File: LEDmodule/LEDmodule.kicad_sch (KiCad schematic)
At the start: 2 parts

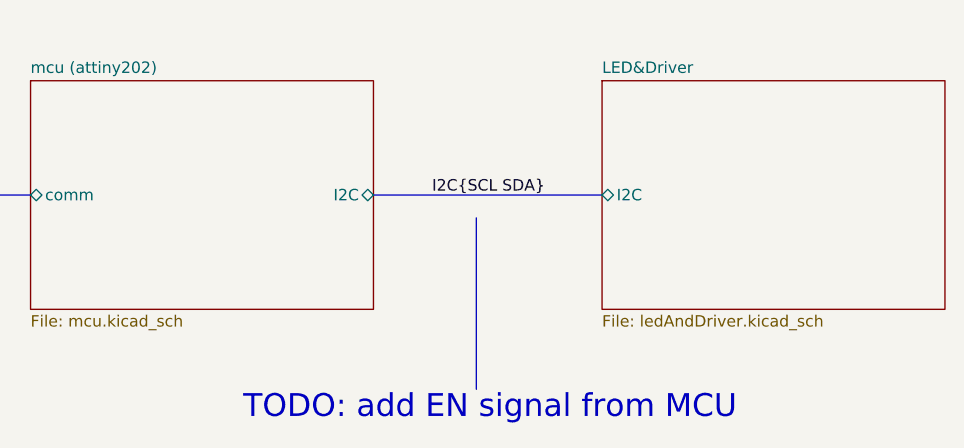
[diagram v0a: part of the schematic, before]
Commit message: Finalize Led&Driver
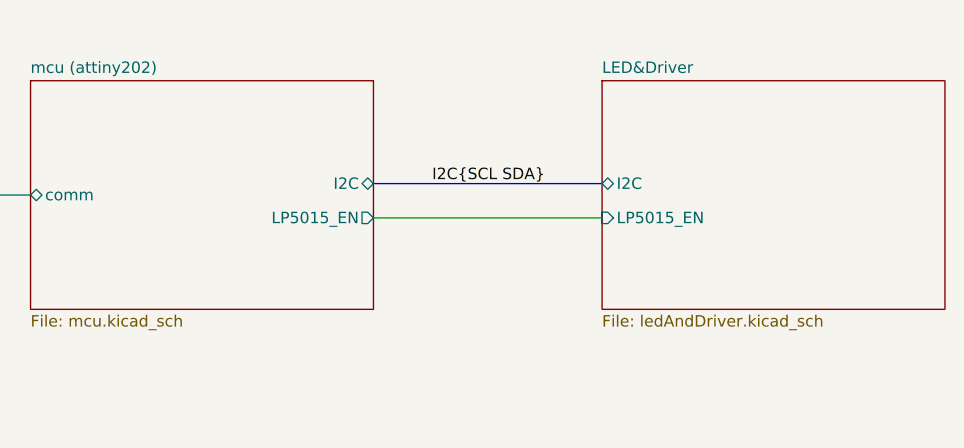
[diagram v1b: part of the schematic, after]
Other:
- sheet LED&Driver ports: added LP5015_EN; removed none
- sheet mcu (attiny202) ports: added LP5015_EN; removed none
- note removed: "TODO: add EN signal from MCU"
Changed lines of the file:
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@@
 		(comment 1 "${Designed By}")
-	)
-	(text "TODO: add EN signal from MCU"
-		(exclude_from_sim no)
-		(at 228.854 150.622 0)
-		(effects
-			(font
-				(size 2.54 2.54)
-				(color 255 0 0 1)
-			)
-		)
 	)
 	(junction
@@
 	(bus
 		(pts
-			(xy 215.9 127) (xy 241.3 127)
+			(xy 215.9 125.73) (xy 241.3 125.73)
 		)
 		(stroke
@@
 		)
 	)
-	(polyline
-		(pts
-			(xy 227.33 129.54) (xy 227.33 148.59)
-		)
-		(stroke
-			(width 0)
-			(type solid)
-			(color 255 0 0 1)
-		)
-	)
 	(wire
 		(pts
@@
 	(wire
 		(pts
+			(xy 215.9 129.54) (xy 241.3 129.54)
+		)
+		(stroke
+			(width 0)
+			(type default)
+		)
+	)
+	(wire
+		(pts
 			(xy 101.6 82.55) (xy 101.6 120.65)
 		)
@@
 	)
 	(label "I2C{SCL SDA}"
-		(at 234.95 127 180)
+		(at 234.95 125.73 180)
 		(effects
 			(font
@@
 		)
 		(pin "I2C" bidirectional
-			(at 215.9 127 0)
+			(at 215.9 125.73 0)
+			(effects
+				(font
+					(size 1.27 1.27)
+				)
+				(justify right)
+			)
+		)
+		(pin "LP5015_EN" output
+			(at 215.9 129.54 0)
 			(effects
 				(font
@@
 		)
 		(pin "I2C" bidirectional
-			(at 241.3 127 180)
-			(effects
-				(font
+			(at 241.3 125.73 180)
+			(effects
+				(font
+					(size 1.27 1.27)
+				)
+				(justify left)
+			)
+		)
+		(pin "LP5015_EN" input
+			(at 241.3 129.54 180)
+			(effects
+				(font
